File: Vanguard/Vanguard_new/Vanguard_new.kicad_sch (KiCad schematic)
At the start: 72 parts, among them J1 USB_C, J2 Conn_02x03_Pin, J3 Micro_SD_Card_Det1, J4 STARBOARD_SERVO, J5 PORTSIDE_SERVO, J6 Conn_01x02_Pin, Q1 BSS138, Q2 BSS138, Q3 BSS138, Q4 BSS138, U1 ATSAMD11D14A-M, U2 ATmega4809-A, U3 AT25DF641A-SH-T, U4 AP2112K-3.3, U5 MPM3610AGQV-P, U6 BNO086, U7 TXB0104D, U8 TPS61092, Y1 32.768kHz

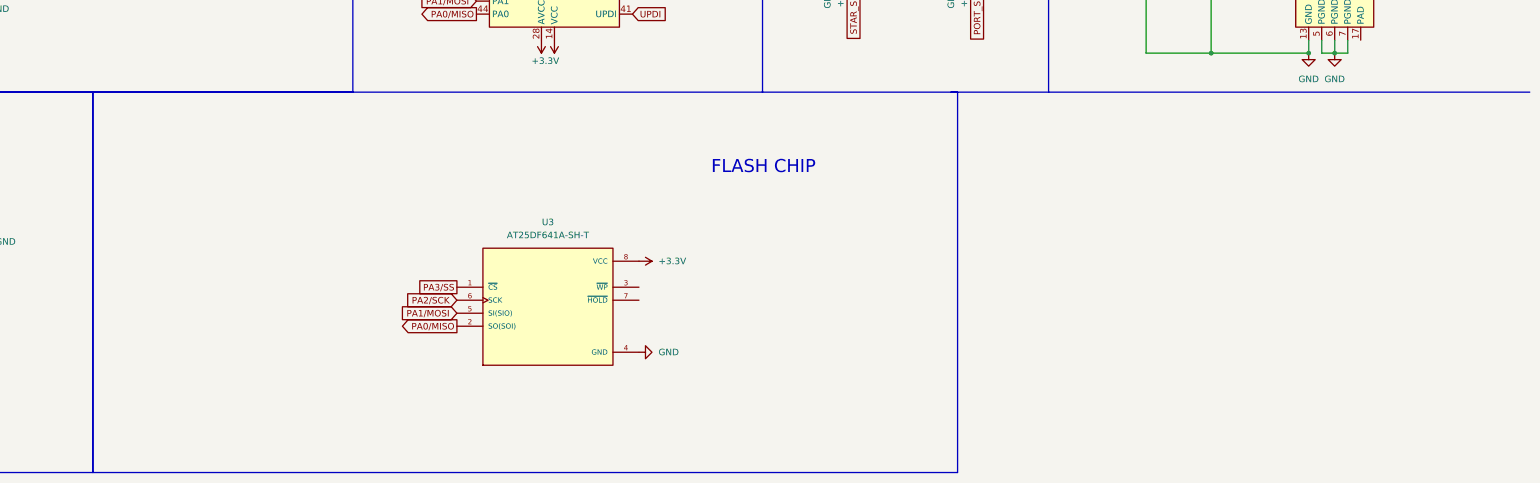
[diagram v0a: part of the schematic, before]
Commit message: small changes
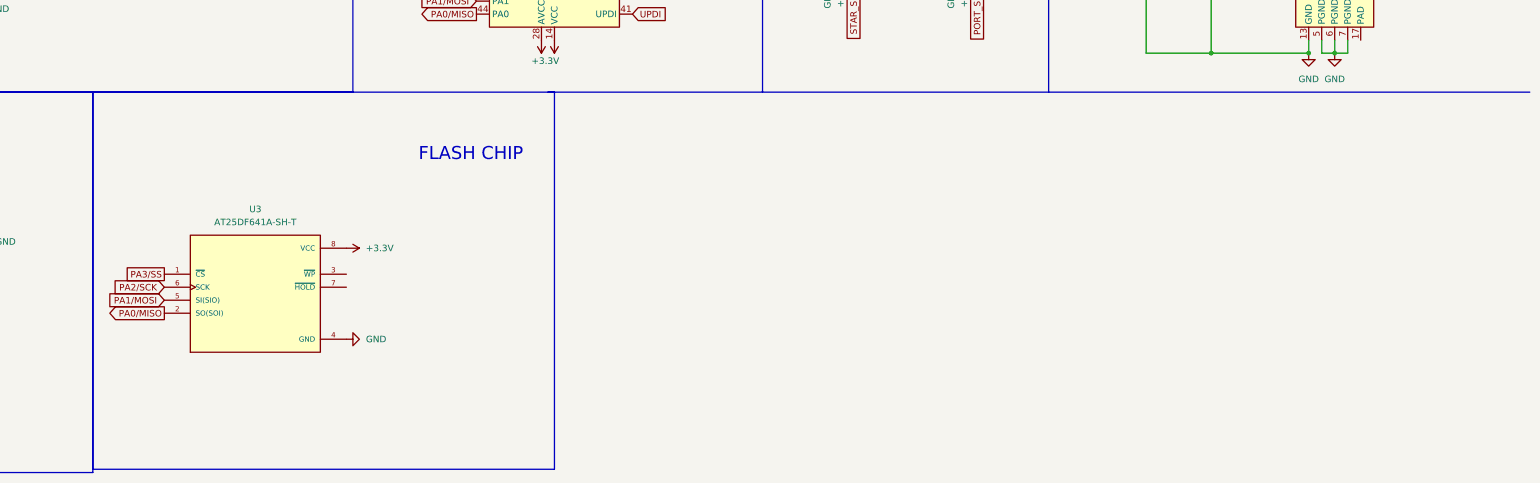
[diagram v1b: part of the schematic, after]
